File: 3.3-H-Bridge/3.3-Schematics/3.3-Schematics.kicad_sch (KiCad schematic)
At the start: 4 parts, among them M1 Motor_DC, SW1 SW_Push, U1 SN754410NE

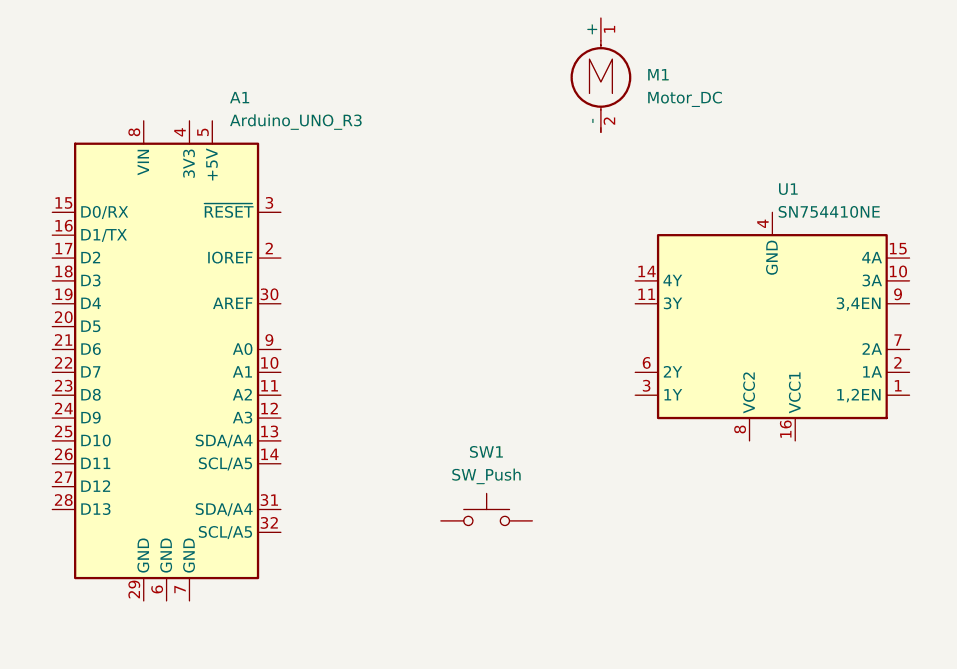
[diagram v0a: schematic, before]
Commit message: schematics
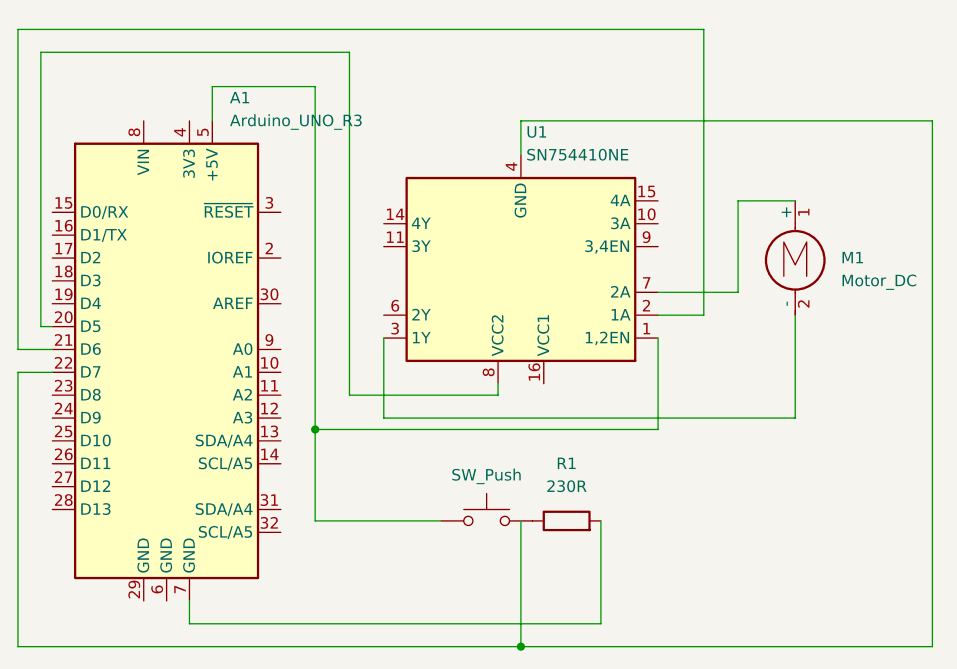
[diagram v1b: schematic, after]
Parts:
- added R1: 230R, symbol Device:R
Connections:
- net at M1.1 (+): now also U1.7 (2A)
- net at M1.2 (-): now also U1.3 (1Y)
- net at A1.20 (D5): now also U1.8 (VCC2)
- net at A1.21 (D6): now also U1.2 (1A)
- net at A1.22 (D7): now also U1.12 (GND), U1.13 (GND), U1.4 (GND), U1.5 (GND)
- net at A1.5 (+5V): now also SW1.1, U1.1 (1,2EN)
- net at A1.7 (GND): now also R1.2
- net at SW1.2: now also R1.1
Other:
- moved on the sheet: M1, U1
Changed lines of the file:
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@@
 (kicad_sch (version 20230121) (generator eeschema)
   (paper "A4")
-  (symbol (lib_id "Motor:Motor_DC") (at 167.64 60.96 0) (unit 1)
-    (in_bom yes) (on_board yes) (dnp no) (fields_autoplaced)
-    (property "Reference" "M1" (at 172.72 62.23 0)
-      (effects (font (size 1.27 1.27)) (justify left))
-    )
-    (property "Value" "Motor_DC" (at 172.72 64.77 0)
-      (effects (font (size 1.27 1.27)) (justify left))
-    )
-    (property "Footprint" "" (at 167.64 63.246 0)
-      (effects (font (size 1.27 1.27)) hide)
-    )
-    (property "Datasheet" "~" (at 167.64 63.246 0)
+  (junction (at 158.75 125.73) (diameter 0) (color 0 0 0 0)
+  )
+  (junction (at 135.89 101.6) (diameter 0) (color 0 0 0 0)
+  )
+  (wire (pts (xy 182.88 76.2) (xy 189.23 76.2))
+    (stroke (width 0) (type default))
+  )
+  (wire (pts (xy 121.92 123.19) (xy 167.64 123.19))
+    (stroke (width 0) (type default))
+  )
+  (wire (pts (xy 143.51 100.33) (xy 189.23 100.33))
+    (stroke (width 0) (type default))
+  )
+  (wire (pts (xy 105.41 90.17) (xy 106.68 90.17))
+    (stroke (width 0) (type default))
+  )
+  (wire (pts (xy 106.68 95.25) (xy 102.87 95.25))
+    (stroke (width 0) (type default))
+  )
+  (wire (pts (xy 102.87 125.73) (xy 158.75 125.73))
+    (stroke (width 0) (type default))
+  )
+  (wire (pts (xy 179.07 88.9) (xy 179.07 57.15))
+    (stroke (width 0) (type default))
+  )
+  (wire (pts (xy 204.47 125.73) (xy 158.75 125.73))
+    (stroke (width 0) (type default))
+  )
+  (wire (pts (xy 173.99 86.36) (xy 182.88 86.36))
+    (stroke (width 0) (type default))
+  )
+  (wire (pts (xy 105.41 59.69) (xy 105.41 90.17))
+    (stroke (width 0) (type default))
+  )
+  (wire (pts (xy 102.87 95.25) (xy 102.87 125.73))
+    (stroke (width 0) (type default))
+  )
+  (wire (pts (xy 173.99 91.44) (xy 173.99 101.6))
+    (stroke (width 0) (type default))
+  )
+  (wire (pts (xy 135.89 101.6) (xy 173.99 101.6))
+    (stroke (width 0) (type default))
+  )
+  (wire (pts (xy 135.89 63.5) (xy 135.89 101.6))
+    (stroke (width 0) (type default))
+  )
+  (wire (pts (xy 139.7 97.79) (xy 139.7 59.69))
+    (stroke (width 0) (type default))
+  )
+  (wire (pts (xy 102.87 57.15) (xy 102.87 92.71))
+    (stroke (width 0) (type default))
+  )
+  (wire (pts (xy 135.89 111.76) (xy 149.86 111.76))
+    (stroke (width 0) (type default))
+  )
+  (wire (pts (xy 143.51 91.44) (xy 143.51 100.33))
+    (stroke (width 0) (type default))
+  )
+  (wire (pts (xy 156.21 97.79) (xy 139.7 97.79))
+    (stroke (width 0) (type default))
+  )
+  (wire (pts (xy 158.75 67.31) (xy 204.47 67.31))
+    (stroke (width 0) (type default))
+  )
+  (wire (pts (xy 156.21 96.52) (xy 156.21 97.79))
+    (stroke (width 0) (type default))
+  )
+  (wire (pts (xy 158.75 71.12) (xy 158.75 67.31))
+    (stroke (width 0) (type default))
+  )
+  (wire (pts (xy 173.99 88.9) (xy 179.07 88.9))
+    (stroke (width 0) (type default))
+  )
+  (wire (pts (xy 121.92 120.65) (xy 121.92 123.19))
+    (stroke (width 0) (type default))
+  )
+  (wire (pts (xy 158.75 111.76) (xy 158.75 125.73))
+    (stroke (width 0) (type default))
+  )
+  (wire (pts (xy 204.47 67.31) (xy 204.47 125.73))
+    (stroke (width 0) (type default))
+  )
+  (wire (pts (xy 189.23 100.33) (xy 189.23 88.9))
+    (stroke (width 0) (type default))
+  )
+  (wire (pts (xy 182.88 86.36) (xy 182.88 76.2))
+    (stroke (width 0) (type default))
+  )
+  (wire (pts (xy 139.7 59.69) (xy 105.41 59.69))
+    (stroke (width 0) (type default))
+  )
+  (wire (pts (xy 124.46 67.31) (xy 124.46 63.5))
+    (stroke (width 0) (type default))
+  )
+  (wire (pts (xy 179.07 57.15) (xy 102.87 57.15))
+    (stroke (width 0) (type default))
+  )
+  (wire (pts (xy 102.87 92.71) (xy 106.68 92.71))
+    (stroke (width 0) (type default))
+  )
+  (wire (pts (xy 124.46 63.5) (xy 135.89 63.5))
+    (stroke (width 0) (type default))
+  )
+  (wire (pts (xy 167.64 111.76) (xy 167.64 123.19))
+    (stroke (width 0) (type default))
+  )
+  (wire (pts (xy 135.89 101.6) (xy 135.89 111.76))
+    (stroke (width 0) (type default))
+  )
+  (symbol (lib_id "Motor:Motor_DC") (at 189.23 81.28 0) (unit 1)
+    (in_bom yes) (on_board yes) (dnp no) (fields_autoplaced)
+    (property "Reference" "M1" (at 194.31 82.55 0)
+      (effects (font (size 1.27 1.27)) (justify left))
+    )
+    (property "Value" "Motor_DC" (at 194.31 85.09 0)
+      (effects (font (size 1.27 1.27)) (justify left))
+    )
+    (property "Footprint" "" (at 189.23 83.566 0)
+      (effects (font (size 1.27 1.27)) hide)
+    )
+    (property "Datasheet" "~" (at 189.23 83.566 0)
       (effects (font (size 1.27 1.27)) hide)
     )
@@
     )
   )
-  (symbol (lib_id "Driver_Motor:SN754410NE") (at 186.69 90.17 180) (unit 1)
-    (in_bom yes) (on_board yes) (dnp no) (fields_autoplaced)
-    (property "Reference" "U1" (at 187.2741 74.93 0)
+  (symbol (lib_id "Device:R") (at 163.83 111.76 90) (unit 1)
+    (in_bom yes) (on_board yes) (dnp no) (fields_autoplaced)
+    (property "Reference" "R1" (at 163.83 105.41 90)
+      (effects (font (size 1.27 1.27)))
+    )
+    (property "Value" "230R" (at 163.83 107.95 90)
+      (effects (font (size 1.27 1.27)))
+    )
+    (property "Footprint" "" (at 163.83 113.538 90)
+      (effects (font (size 1.27 1.27)) hide)
+    )
+    (property "Datasheet" "~" (at 163.83 111.76 0)
+      (effects (font (size 1.27 1.27)) hide)
+    )
+    (pin "1")
+    (pin "2")
+    (instances
+      (project "3.3-Schematics"
+        (path "/1e8ab3d7-208c-45ee-8224-191a416a7e09"
+          (reference "R1") (unit 1)
+        )
+      )
+    )
+  )
+  (symbol (lib_id "Driver_Motor:SN754410NE") (at 158.75 83.82 180) (unit 1)
+    (in_bom yes) (on_board yes) (dnp no) (fields_autoplaced)
+    (property "Reference" "U1" (at 159.3341 68.58 0)
       (effects (font (size 1.27 1.27)) (justify right))
     )
-    (property "Value" "SN754410NE" (at 187.2741 77.47 0)
+    (property "Value" "SN754410NE" (at 159.3341 71.12 0)
       (effects (font (size 1.27 1.27)) (justify right))
     )
-    (property "Footprint" "Package_DIP:DIP-16_W7.62mm" (at 189.23 113.03 0)
-      (effects (font (size 1.27 1.27)) hide)
-    )
-    (property "Datasheet" "https://www.ti.com/lit/ds/symlink/sn754410.pdf" (at 186.69 115.57 0)
+    (property "Footprint" "Package_DIP:DIP-16_W7.62mm" (at 161.29 106.68 0)
+      (effects (font (size 1.27 1.27)) hide)
+    )
+    (property "Datasheet" "https://www.ti.com/lit/ds/symlink/sn754410.pdf" (at 158.75 109.22 0)
       (effects (font (size 1.27 1.27)) hide)
     )
@@
     (in_bom yes) (on_board yes) (dnp no) (fields_autoplaced)
     (property "Reference" "SW1" (at 154.94 104.14 0)
-      (effects (font (size 1.27 1.27)))
+      (effects (font (size 1.27 1.27)) hide)
     )
     (property "Value" "SW_Push" (at 154.94 106.68 0)
